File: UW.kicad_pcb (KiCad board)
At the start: 2 copper layers, 19.9 x 26.5 mm, 43 parts, among them J1 SH1.0, J2 SH1.0, J3 USB_C_Receptacle_PowerOnly_6P, Q1 AO3401A, Q2 MBT3904DW1, SW1 Reset, SW2 Boot, SW3 SW_SPDT, U1 AP2112K-3.3, U2 ESP32-WROOM-32U, U3 MCP73831-2-OT, U4 MPU-6050

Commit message: Update Board
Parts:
- moved G*** 0.21 mm to (103.7, 35.5)

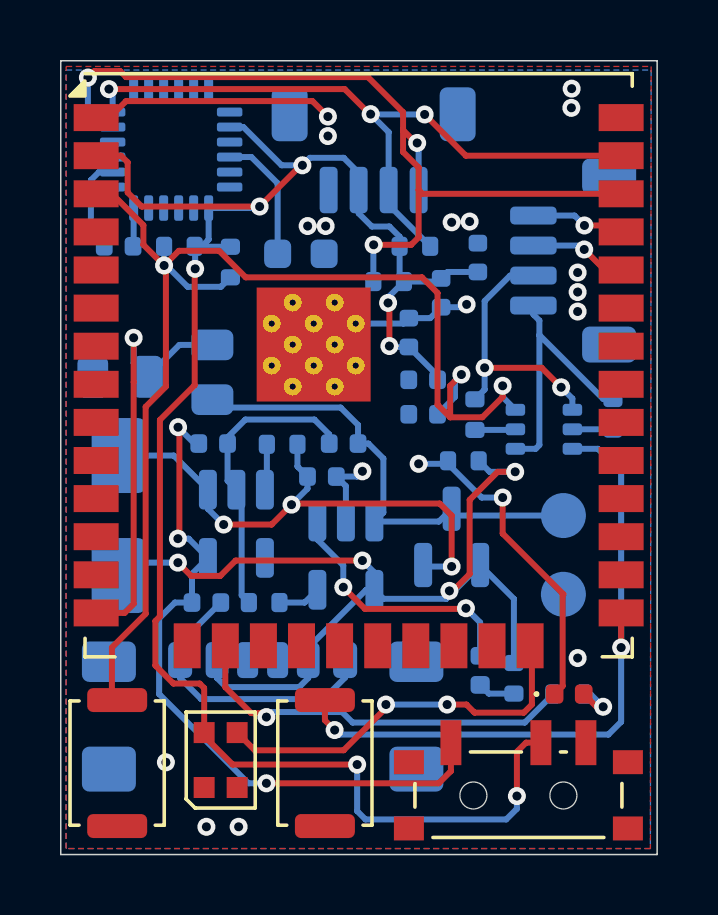
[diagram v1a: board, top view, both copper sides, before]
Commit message: Update UW.kicad_pcb
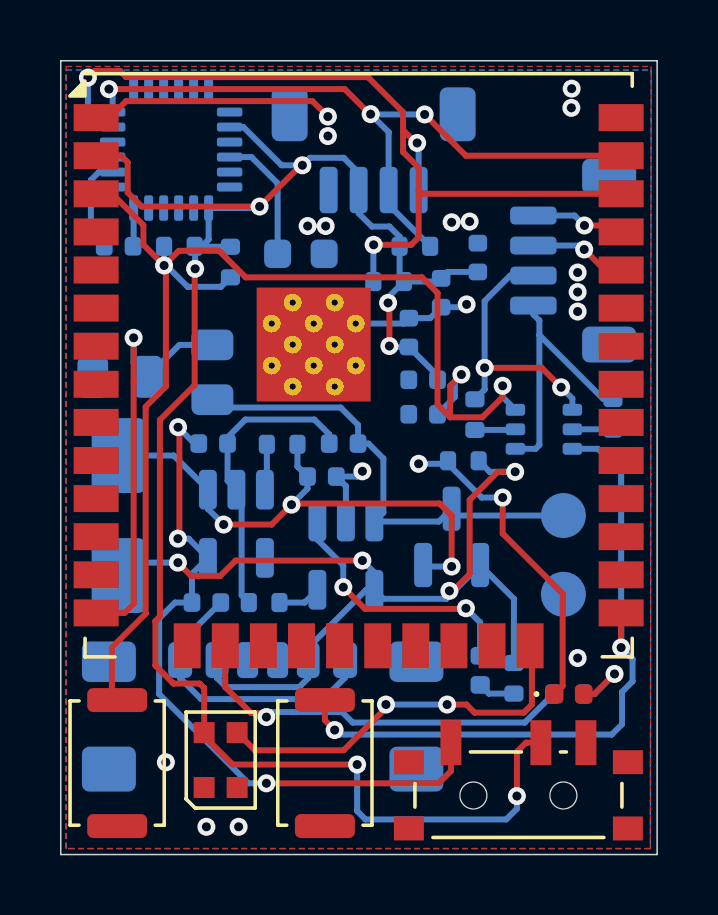
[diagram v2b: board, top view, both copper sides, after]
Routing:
- net Net-(D4-A): track 1.64 -> 2.60 mm
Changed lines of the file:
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@@
 	)
 	(segment
-		(start 106.25 55.453486)
-		(end 106.025986 55.453486)
+		(start 106.63 54.36)
+		(end 105.96 55.03)
 		(width 0.2)
 		(layer "F.Cu")
@@
 	)
 	(segment
-		(start 106.025986 55.453486)
+		(start 105.96 55.03)
 		(end 105.6025 55.03)
 		(width 0.2)
@@
 	)
 	(via
-		(at 106.25 55.453486)
+		(at 106.63 54.36)
 		(size 0.6)
 		(drill 0.3)
@@
 	)
 	(segment
-		(start 105.826514 55.03)
-		(end 106.25 55.453486)
+		(start 105.96 55.03)
+		(end 105.61 55.03)
 		(width 0.2)
 		(layer "B.Cu")
@@
 	)
 	(segment
-		(start 105.61 55.03)
-		(end 105.826514 55.03)
+		(start 106.63 54.36)
+		(end 105.96 55.03)
 		(width 0.2)
 		(layer "B.Cu")
@@
 	)
 	(segment
-		(start 106.85 55.955)
-		(end 106.85 53.48)
+		(start 107.23 54.608529)
+		(end 107.23 53.86)
 		(width 0.2)
 		(layer "B.Cu")
@@
 	)
 	(segment
+		(start 107.23 53.86)
+		(end 106.85 53.48)
+		(width 0.2)
+		(layer "B.Cu")
+		(net 22)
+	)
+	(segment
+		(start 106.54 56.38)
+		(end 106.88 56.04)
+		(width 0.2)
+		(layer "B.Cu")
+		(net 22)
+	)
+	(segment
 		(start 105.225 46.855)
 		(end 106.075 46.855)
@@
 	)
 	(segment
+		(start 106.88 56.04)
+		(end 106.88 54.958529)
+		(width 0.2)
+		(layer "B.Cu")
+		(net 22)
+	)
+	(segment
 		(start 106.85 53.48)
 		(end 106.85 52.325)
@@
 	)
 	(segment
+		(start 97.3 56.23)
+		(end 97.45 56.38)
+		(width 0.2)
+		(layer "B.Cu")
+		(net 22)
+	)
+	(segment
+		(start 97.45 56.38)
+		(end 106.54 56.38)
+		(width 0.2)
+		(layer "B.Cu")
+		(net 22)
+	)
+	(segment
 		(start 106.85 47.63)
 		(end 106.85 52.325)
@@
 	)
 	(segment
-		(start 97.3 56.23)
-		(end 97.45 56.38)
-		(width 0.2)
-		(layer "B.Cu")
-		(net 22)
-	)
-	(segment
-		(start 97.45 56.38)
-		(end 106.425 56.38)
-		(width 0.2)
-		(layer "B.Cu")
-		(net 22)
-	)
-	(segment
-		(start 106.425 56.38)
-		(end 106.85 55.955)
-		(width 0.2)
-		(layer "B.Cu")
+		(start 106.88 54.958529)
+		(end 107.23 54.608529)
+		(width 0.2)
+		(layer "B.Cu")
